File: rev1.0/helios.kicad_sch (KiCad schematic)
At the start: 54 parts, among them J1 USB_C_Receptacle_USB2.0, J2 helios-pinout, Q1 2N7002VC-, Q2 2N7002VC-, SW1 SWITCH, U1 USBLC6-2P6, U2 LP5907SNX-3.3-NOPB, U3 W25Q128JVPIQ, U4 RP2040, U5 74LVC1T45, Y1 12MHz

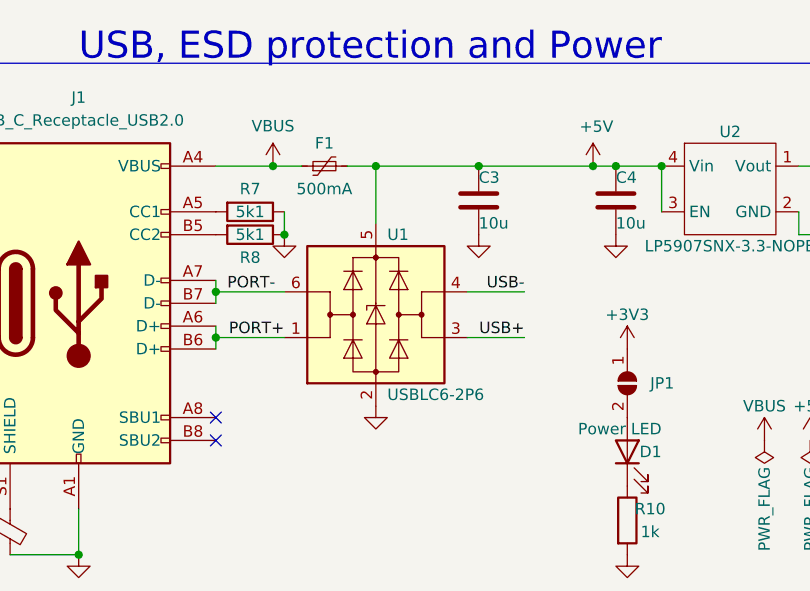
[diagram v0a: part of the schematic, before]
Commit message: added prod files for jlcpcb
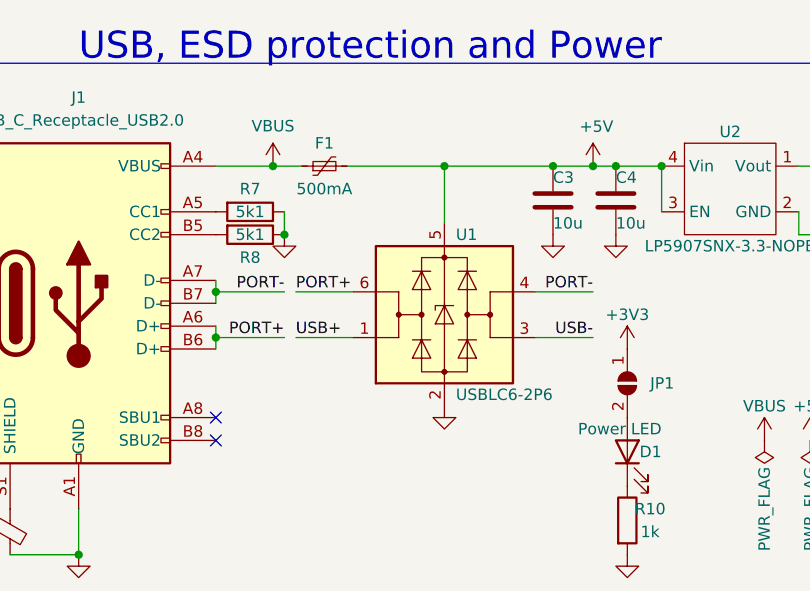
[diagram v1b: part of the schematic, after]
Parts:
- J2, JP1: now left out of the parts list
- Q1, Q2: JLCPCB_CORRECTION (none) -> 0; 0; 180
- U1, U2, U3, U5: JLCPCB_CORRECTION (none) -> 0; 0; 270
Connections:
- net PORT+: now also U1.6 (I/O1); no longer U1.1 (I/O1)
- net PORT-: now also U1.4 (I/O2); no longer U1.6 (I/O1)
- net USB+: now also U1.1 (I/O1); no longer U1.3 (I/O2)
- net USB-: now also U1.3 (I/O2); no longer U1.4 (I/O2)
